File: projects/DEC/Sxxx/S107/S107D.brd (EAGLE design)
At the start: 125.7 x 62.2 mm, 64 parts, among them Q1 2N3639, Q2 2N3639, Q3 2N3639, Q4 2N3639, Q5 2N3639, Q6 2N3639, Q7 2N3639

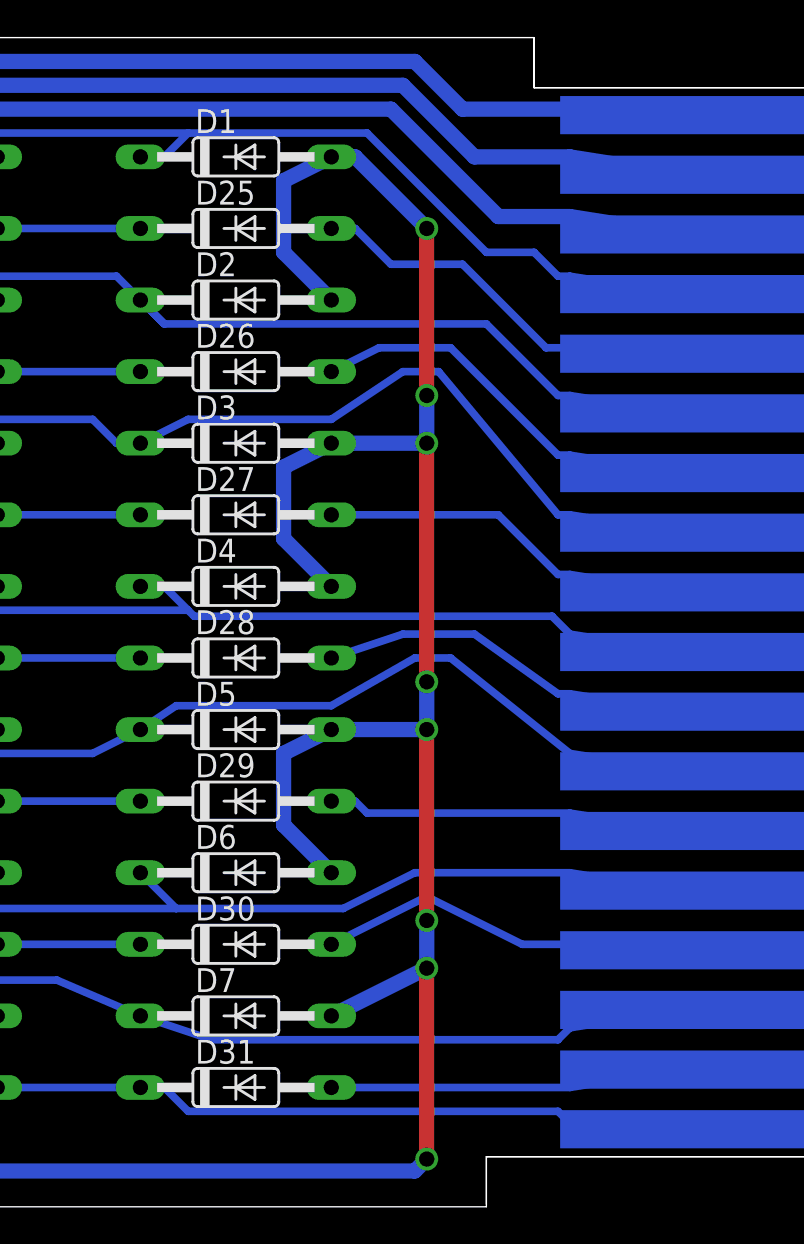
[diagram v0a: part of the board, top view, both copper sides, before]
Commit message: Walk the project tree, making things pass current design rules.
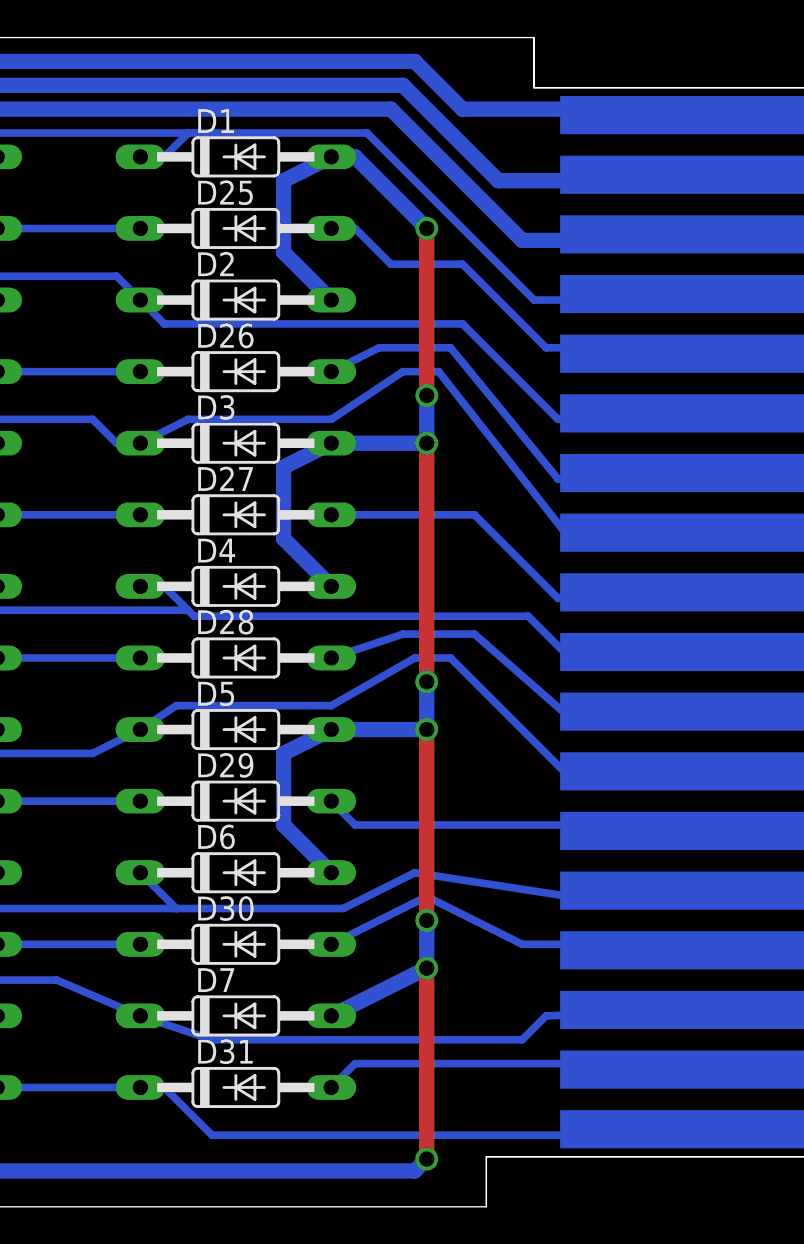
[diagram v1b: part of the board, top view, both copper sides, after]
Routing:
- net N$4: track 84.3 -> 82.9 mm
- net N$5: track 21.5 -> 22.4 mm
- net N$30: track 84.9 -> 85.7 mm
- net N$9: track 84.9 -> 85.6 mm
- net N$26: track 20.0 -> 20.6 mm
